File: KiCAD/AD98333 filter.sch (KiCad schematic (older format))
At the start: 1 part

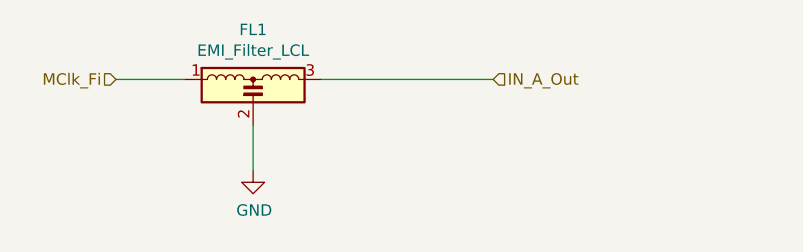
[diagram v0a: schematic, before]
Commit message: Schematics and PCB update
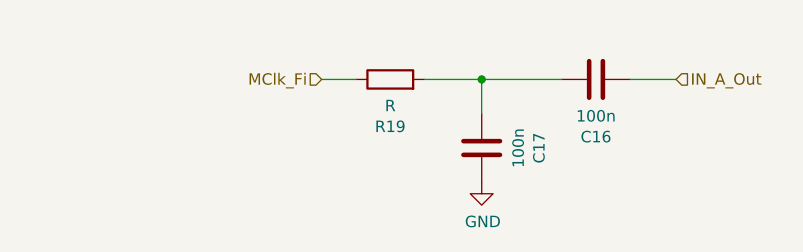
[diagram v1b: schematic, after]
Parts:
- removed FL1: EMI_Filter_LCL, Ceramic_Filter:SFECK, symbol Device:EMI_Filter_LCL
- added C16, C17: 100n, Capacitor_SMD:C_0805_2012Metric, symbol Device:C
- added R19: R, Resistor_SMD:R_0805_2012Metric, symbol Device:R
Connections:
- net GND: now also C17.1
- net IN_A_Out: now also C16.2
- net MClk_Fi: now also R19.1
- new net: C16.1, C17.2, R19.2
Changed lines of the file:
@@
 Comment4 ""
 $EndDescr
+Text HLabel 5300 1650 2    50   Input ~ 0
+IN_A_Out
 $Comp
-L Device:EMI_Filter_LCL FL1
-U 1 1 5E7CF349
-P 3450 1750
-F 0 "FL1" H 3450 2067 50  0000 C CNN
-F 1 "EMI_Filter_LCL" H 3450 1976 50  0000 C CNN
-F 2 "Ceramic_Filter:SFECK" V 3450 1750 50  0001 C CNN
-F 3 "http://www.murata.com/~/media/webrenewal/support/library/catalog/products/emc/emifil/c31e.ashx?la=en-gb" V 3450 1750 50  0001 C CNN
-	1    3450 1750
-	1    0    0    -1
+L Device:C C?
+U 1 1 5E9AE17E
+P 4950 1650
+AR Path="/5E70F6BF/5E9AE17E" Ref="C?"  Part="1"
+AR Path="/5E9AE17E" Ref="C?"  Part="1"
+AR Path="/5E71DA61/5E9AE17E" Ref="C16"  Part="1"
+F 0 "C16" V 4698 1650 50  0000 C CNN
+F 1 "100n" V 4789 1650 50  0000 C CNN
+F 2 "Capacitor_SMD:C_0805_2012Metric" H 4988 1500 50  0001 C CNN
+F 3 "~" H 4950 1650 50  0001 C CNN
+	1    4950 1650
+	0    -1   -1   0
 $EndComp
 $Comp
-L power:GND #PWR0128
-U 1 1 5E7CF8C3
-P 3450 2050
-F 0 "#PWR0128" H 3450 1800 50  0001 C CNN
-F 1 "GND" H 3455 1877 50  0000 C CNN
-F 2 "" H 3450 2050 50  0001 C CNN
-F 3 "" H 3450 2050 50  0001 C CNN
-	1    3450 2050
+L Device:R R?
+U 1 1 5E9B32E8
+P 4050 1650
+AR Path="/5E9B32E8" Ref="R?"  Part="1"
+AR Path="/5E71DA61/5E9B32E8" Ref="R19"  Part="1"
+F 0 "R19" V 3843 1650 50  0000 C CNN
+F 1 "R" V 3934 1650 50  0000 C CNN
+F 2 "Resistor_SMD:R_0805_2012Metric" V 3980 1650 50  0001 C CNN
+F 3 "~" H 4050 1650 50  0001 C CNN
+	1    4050 1650
+	0    -1   -1   0
+$EndComp
+$Comp
+L power:GND #PWR0172
+U 1 1 5E9B3A78
+P 4450 2100
+F 0 "#PWR0172" H 4450 1850 50  0001 C CNN
+F 1 "GND" H 4455 1927 50  0000 C CNN
+F 2 "" H 4450 2100 50  0001 C CNN
+F 3 "" H 4450 2100 50  0001 C CNN
+	1    4450 2100
 	1    0    0    -1
 $EndComp
 Wire Wire Line
-	3450 1850 3450 2050
+	3750 1650 3900 1650
 Wire Wire Line
-	2850 1650 3150 1650
+	4200 1650 4450 1650
 Wire Wire Line
-	3750 1650 4500 1650
-Text HLabel 2850 1650 0    50   Input ~ 0
+	5100 1650 5300 1650
+Wire Wire Line
+	4450 1800 4450 1650
+Connection ~ 4450 1650
+Wire Wire Line
+	4450 1650 4800 1650
+$Comp
+L Device:C C?
+U 1 1 5E9B6BE3
+P 4450 1950
+AR Path="/5E70F6BF/5E9B6BE3" Ref="C?"  Part="1"
+AR Path="/5E9B6BE3" Ref="C?"  Part="1"
+AR Path="/5E71DA61/5E9B6BE3" Ref="C17"  Part="1"
+F 0 "C17" V 4198 1950 50  0000 C CNN
+F 1 "100n" V 4289 1950 50  0000 C CNN
+F 2 "Capacitor_SMD:C_0805_2012Metric" H 4488 1800 50  0001 C CNN
+F 3 "~" H 4450 1950 50  0001 C CNN
+	1    4450 1950
+	-1   0    0    1
+$EndComp
+Text HLabel 3750 1650 0    50   Input ~ 0
 MClk_Fi
-Text HLabel 4500 1650 2    50   Input ~ 0
-IN_A_Out
 $EndSCHEMATC
